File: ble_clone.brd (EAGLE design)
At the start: 109.2 x 68.2 mm, 55 parts, among them CON1 MIKROE_BUS_CONN, IC1 PIC24FV16KM202, IC2 3.3 vreg, IC3 PIC24FV16KM202, K1 AQV254R, K2 AQV254R, K3 AQV254R, K4 AQV254R, X1 MCP3208

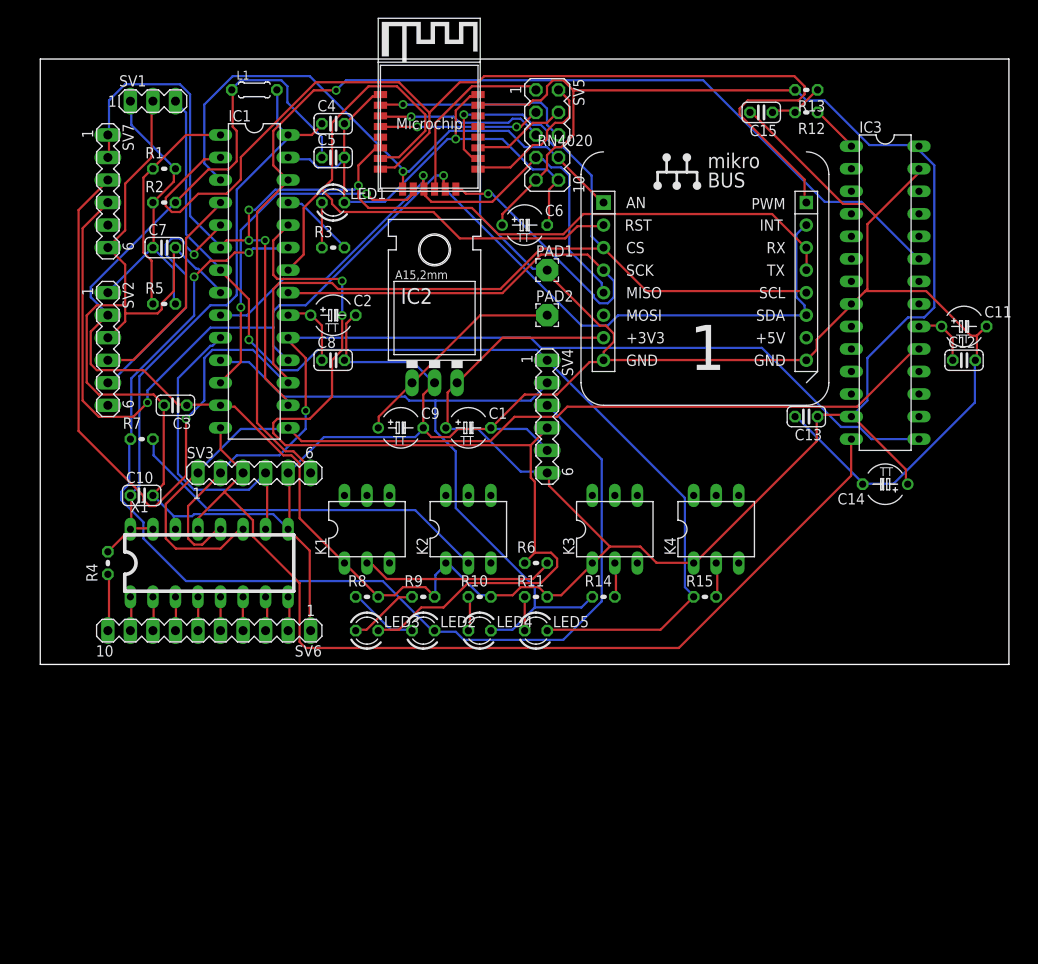
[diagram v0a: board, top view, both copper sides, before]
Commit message: update
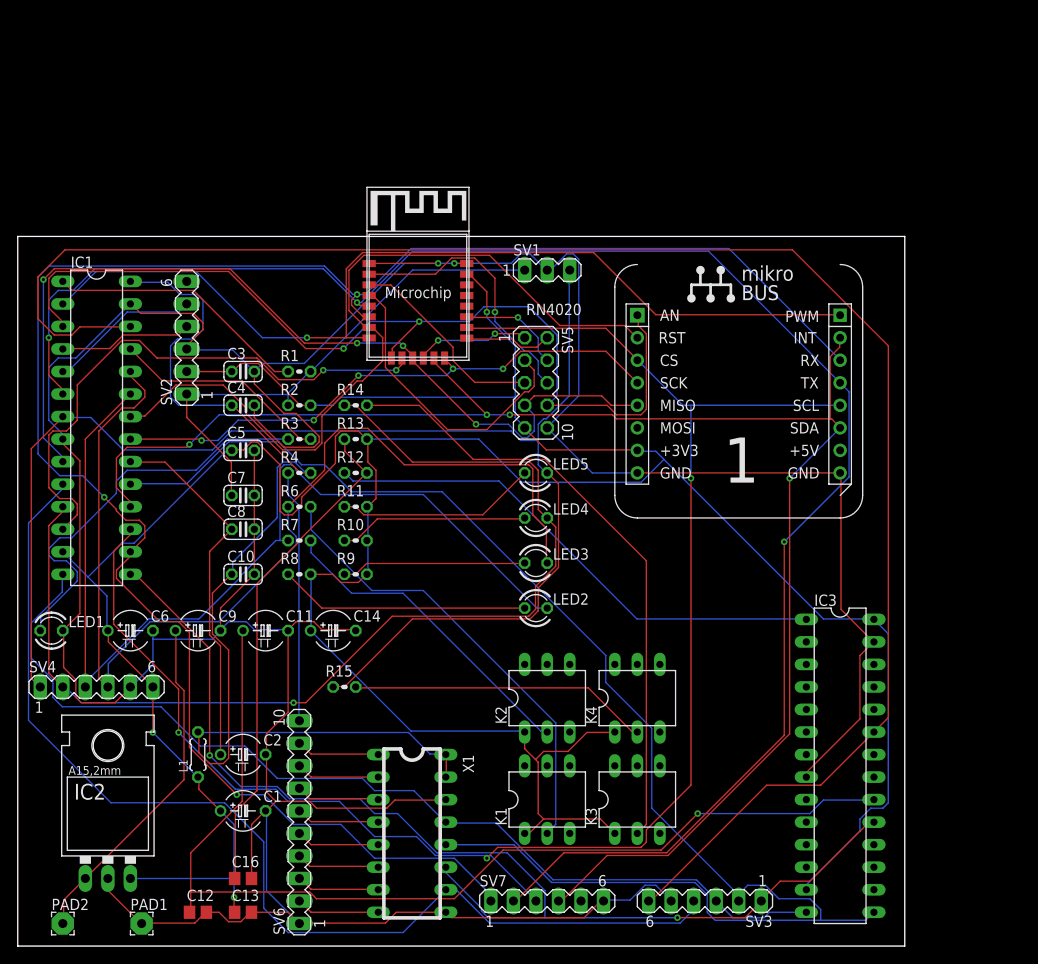
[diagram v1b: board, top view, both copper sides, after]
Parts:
- removed C15: 0.1, resistor:C025-024X044
- removed R5: 470, resistor:0204V
- added C16: 0.1, rcl:C0805
- C12, C13: device resistor:C025-024X044 -> rcl:C0805
- R1: value 470 -> 220
- moved C12 106.4 mm to (20.3, 3.81)
- moved SV7 94.1 mm to (59.7, 5.08), turned to 0 degrees
- moved PAD2 87.7 mm to (5.08, 2.54)
- moved PAD1 86.7 mm to (14.0, 2.54)
- moved C11 85.9 mm to (27.9, 35.6)
- moved C13 84.6 mm to (25.4, 3.81), turned to 0 degrees
- moved L1 75.2 mm to (20.3, 21.6), turned to 90 degrees
- moved SV3 70.1 mm to (77.5, 5.08), turned to 180 degrees
- moved IC2 66.9 mm to (10.2, 11.4)
- moved R12 65.1 mm to (38.1, 53.3), turned to 0 degrees
- moved C14 64.4 mm to (35.6, 35.6), turned to 0 degrees
- moved R13 64.3 mm to (38.1, 57.1), turned to 0 degrees
- moved C6 63.8 mm to (12.7, 35.6)
- moved SV4 59.2 mm to (8.89, 29.2), turned to 0 degrees
- moved LED1 57.8 mm to (3.81, 35.6)
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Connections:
- new net N$4: CON1.P$14, IC1.16, SV7.1, U$1.P06
- net GND: now also C16.2; no longer C15.2
- net N$2: no longer R5.2
- net N$3: no longer CON1.P$14, IC1.16, SV7.1, U$1.P06
- net N$49: now also C16.1; no longer C15.1
- net N$6: no longer R5.1
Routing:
- net N$4: track 0.00 -> 211.6 mm, vias 0 -> 3
- net N$42: track 6.94 -> 116.3 mm, vias 0 -> 1
- net N$18: track 35.4 -> 122.6 mm
- net N$23: track 127.2 -> 195.4 mm, vias 1 -> 0
- net N$44: track 3.89 -> 69.9 mm
- net N$50: track 5.43 -> 58.9 mm
- net N$19: track 112.4 -> 165.6 mm, vias 1 -> 0
- net N$16: track 69.1 -> 121.2 mm
- net N$3: track 143.3 -> 195.0 mm, vias 4 -> 3
- net N$49: track 6.37 -> 56.9 mm
- net N$24: track 80.7 -> 122.4 mm, vias 0 -> 1
- net N$27: track 5.08 -> 46.0 mm
- net N$13: track 67.5 -> 107.4 mm, vias 1 -> 2
- net N$7: track 118.4 -> 157.6 mm, vias 1 -> 0
- net VDD: track 345.7 -> 383.4 mm, vias 0 -> 3
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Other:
- board size 109.2 x 68.2 mm -> 100 x 80 mm
